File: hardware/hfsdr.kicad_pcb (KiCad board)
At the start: 4 copper layers, 100.8 x 73.8 mm, 87 parts, among them J1 USB_C_Receptacle_USB2.0_16P, J4 JST PH S2B, Q1 AO3401A, SW1 RST, SW2 BOOT0, SW8 SW_SPDT, U1 SN74CBT3253, U2 XLV320ADC6120IRTER, U3 CH32V30xRxTx, U4 MD57E33QA3, U5 MD57E33QA3, U6 BGA2817, U7 TP4054, U8 LM4809, X1 2T024000VX, Y1 Si5351A-B-GT

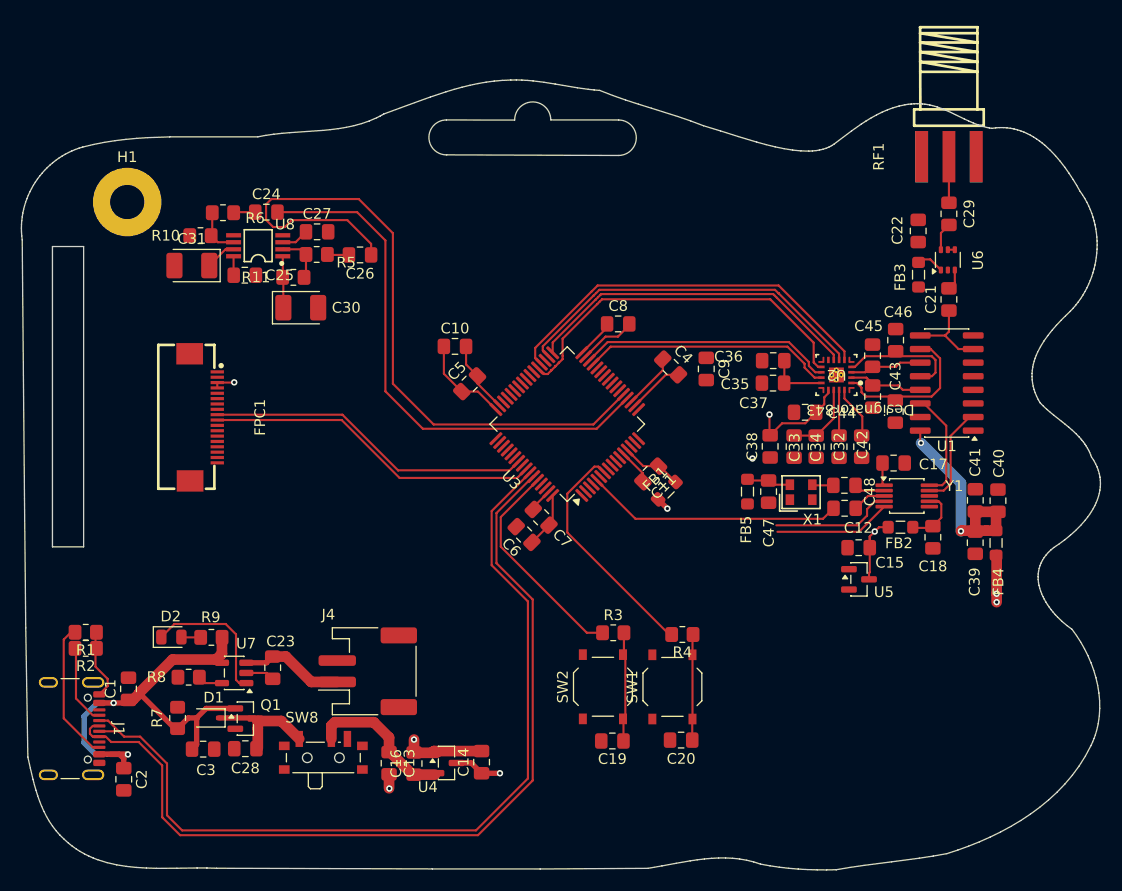
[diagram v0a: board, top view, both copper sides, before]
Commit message: feat: finally got art in
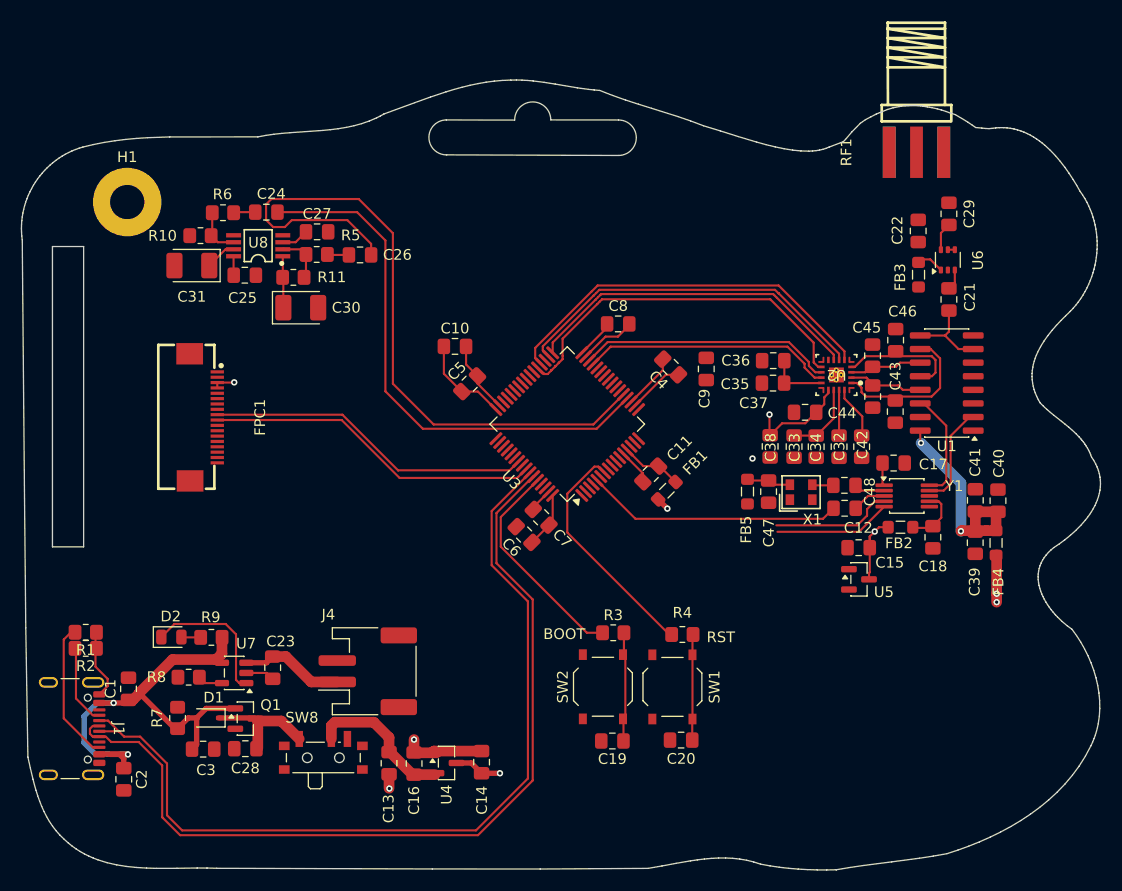
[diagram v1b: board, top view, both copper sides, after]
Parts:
- removed the G*** at (107.9, 67.1)
- removed the G*** at (231.8, 110.8)
- added G***: LOGO, LOGO, B.Cu at (107.7, 67.2)
- moved RF1 3.06 mm to (147.0, 42.6)
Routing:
- net Net-(C29-Pad2): track 4.30 -> 0.00 mm
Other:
- outline, holes or cut-outs redrawn
- board text added: "BOOT"
- board text added: "RST"
